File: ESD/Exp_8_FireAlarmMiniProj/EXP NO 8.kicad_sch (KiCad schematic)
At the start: 6 parts, among them J1 Screw_Terminal_01x02, J2 Screw_Terminal_01x02, U1 LM741

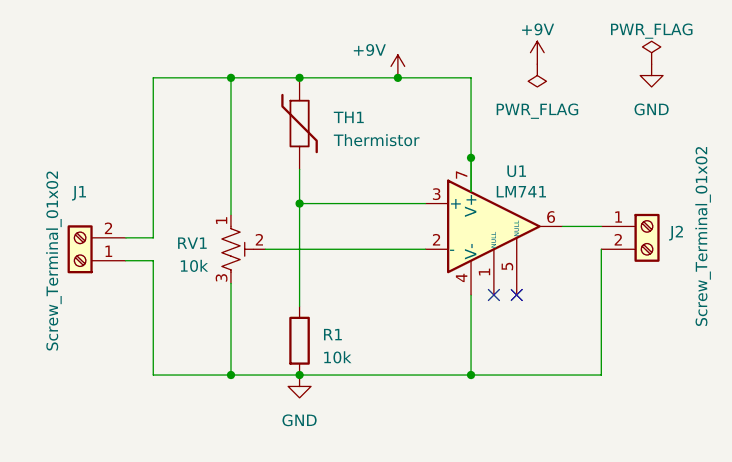
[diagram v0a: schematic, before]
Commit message: Update Eighth Exp in ESD
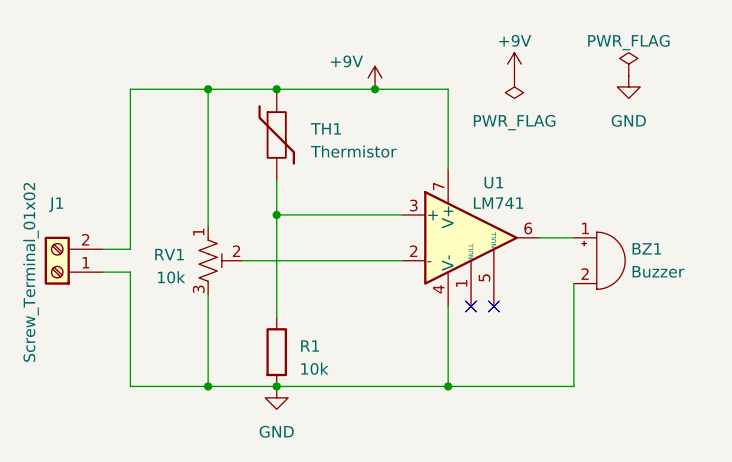
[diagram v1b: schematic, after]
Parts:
- removed J2: Screw_Terminal_01x02, TerminalBlock_Phoenix:TerminalBlock_Phoenix_MKDS-1,5-2-5.08_1x02_P5.08mm_Horizontal, symbol Connector:Screw_Terminal_01x02
- added BZ1: Buzzer, Buzzer_Beeper:Buzzer_12x9.5RM7.6, symbol Device:Buzzer
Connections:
- net GND: now also BZ1.2 (+)
- net at U1.6: now also BZ1.1 (-)
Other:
- moved on the sheet: J1, R1, RV1, TH1, U1
